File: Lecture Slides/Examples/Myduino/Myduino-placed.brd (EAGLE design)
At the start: 66 x 54.3 mm, 30 parts, among them J2 GENERIC-BATTERY-CONN-RECEPTAC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, Y1 16MHz

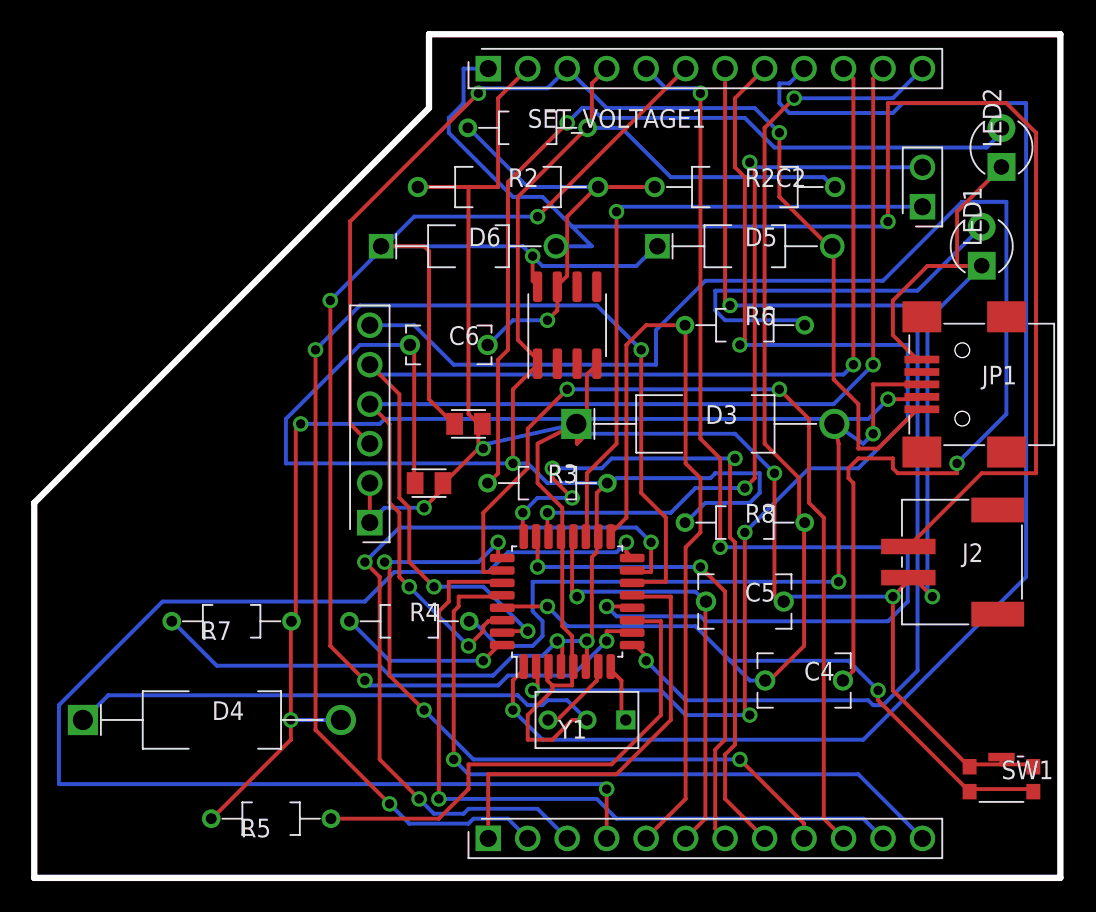
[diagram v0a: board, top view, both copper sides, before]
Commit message: new slides
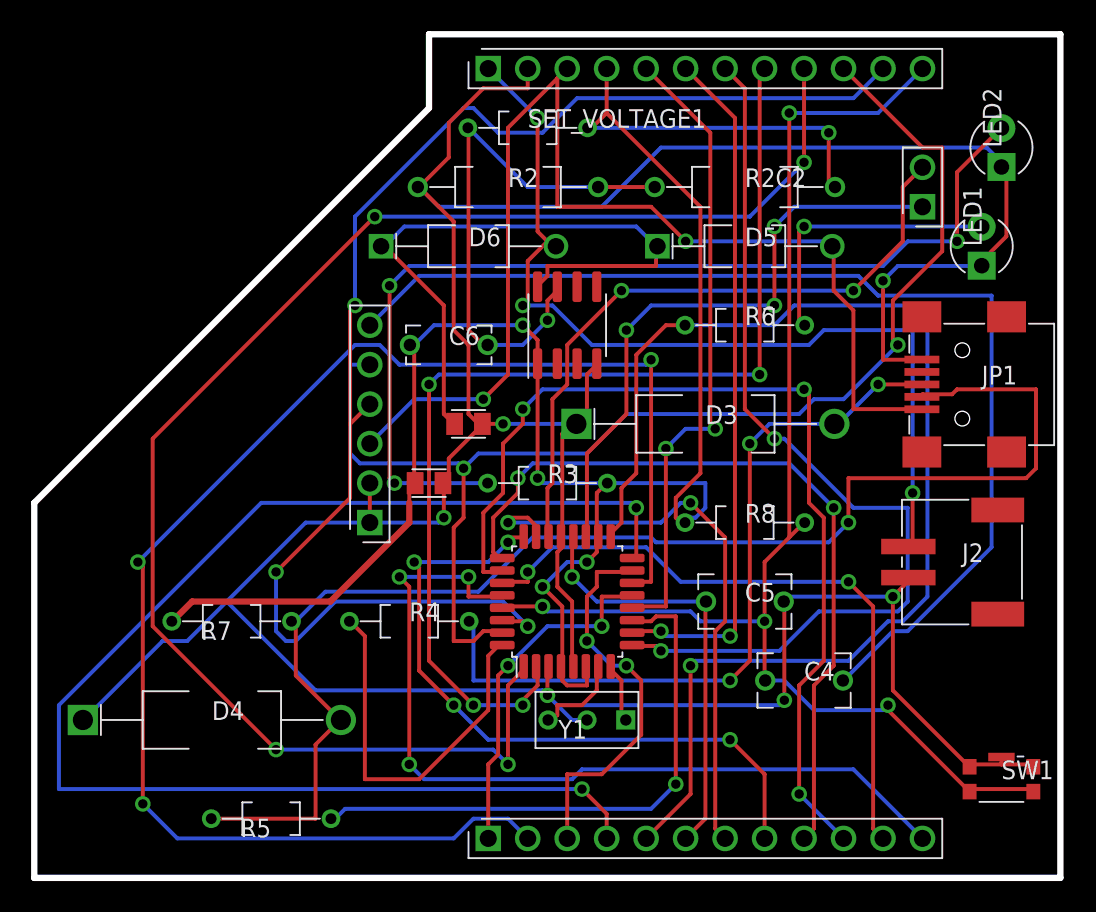
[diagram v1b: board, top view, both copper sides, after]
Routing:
- net VBAT: track 91.1 -> 59.3 mm, vias 1 -> 3
- net D8: track 71.4 -> 41.1 mm, vias 3 -> 2
- net D6: track 73.6 -> 44.4 mm, vias 4 -> 2
- net D13: track 51.9 -> 80.5 mm, vias 0 -> 1
- net D11: track 50.4 -> 25.0 mm, vias 3 -> 2
- net DTR/RTS: track 88.5 -> 71.2 mm, vias 1 -> 0
- net GND: track 215.3 -> 232.4 mm, vias 5 -> 6
- net D-: track 71.9 -> 88.2 mm, vias 3 -> 1
- net RXD: track 74.0 -> 90.0 mm
- net VCC: track 150.2 -> 134.6 mm, vias 3 -> 5
- net D10: track 82.3 -> 97.4 mm
- net D2: track 11.3 -> 25.0 mm, vias 1 -> 0
- net D5: track 72.0 -> 60.9 mm
- net A5: track 45.7 -> 55.7 mm, vias 1 -> 3
- net N$6: track 55.4 -> 65.0 mm, vias 1 -> 3
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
